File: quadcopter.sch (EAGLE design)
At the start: 66 parts, among them J1 ISP, J4 SIP-10_TH-254X10, M1 MOTOR_PADS, M2 MOTOR_PADS, M3 MOTOR_PADS, M4 MOTOR_PADS, U1 ATMEGA128RFA1, Y1 16MHz

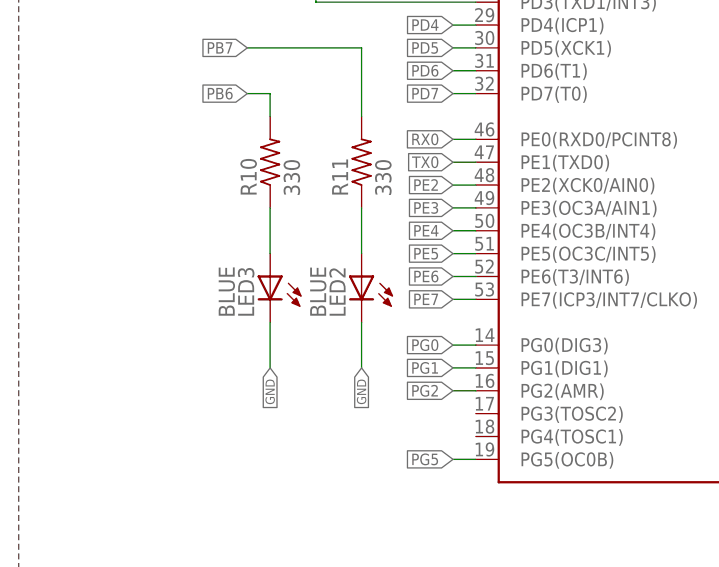
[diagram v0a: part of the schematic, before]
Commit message: Version before generating cam
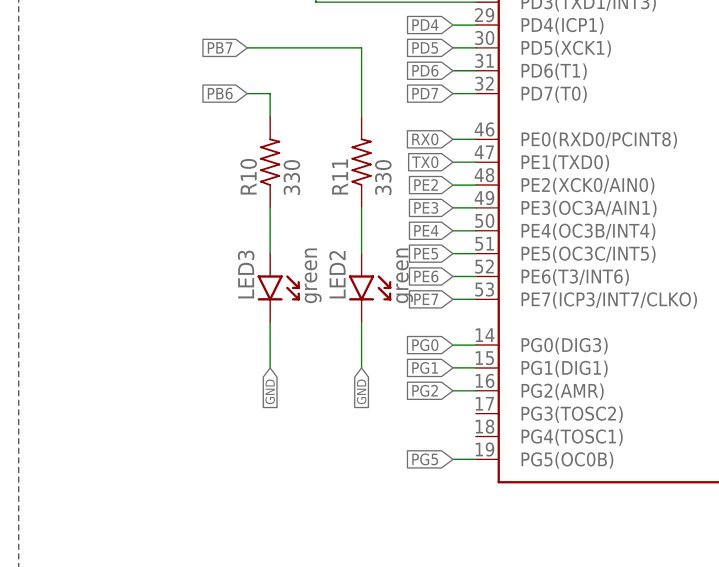
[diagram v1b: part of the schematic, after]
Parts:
- LED2, LED3: value BLUE -> green; device Yueqi Wang-Lab2:LED5MM -> quadparts_prebuilt:DIODE-LED_SMD-2012-0805-GREEN
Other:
- moved on the sheet: LED2, LED3
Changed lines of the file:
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@@
 <part name="JP9" library="quadparts_prebuilt" deviceset="FTDI_BASIC" device="PTH" value="FTDI"/>
 <part name="C16" library="quadparts_prebuilt" deviceset="CAPACITOR-NP_" device="SMD-2012-0805_CERAMIC-0.1UF" value="0.1uF"/>
-<part name="LED2" library="Yueqi Wang-Lab2" deviceset="LED" device="5MM" value="BLUE"/>
+<part name="LED2" library="quadparts_prebuilt" deviceset="DIODE-LED_" device="SMD-2012-0805-GREEN" value="green"/>
 <part name="C17" library="quadparts_prebuilt" deviceset="CAPACITOR-NP_" device="SMD-2012-0805_CERAMIC-0.75PF" value="0.75pF"/>
-<part name="LED3" library="Yueqi Wang-Lab2" deviceset="LED" device="5MM" value="BLUE"/>
+<part name="LED3" library="quadparts_prebuilt" deviceset="DIODE-LED_" device="SMD-2012-0805-GREEN" value="green"/>
 <part name="R10" library="quadparts_prebuilt" deviceset="RESISTOR_" device="SMD-2012-0805-330" value="330"/>
 <part name="R11" library="quadparts_prebuilt" deviceset="RESISTOR_" device="SMD-2012-0805-330" value="330"/>
@@
 <instance part="JP9" gate="G$1" x="38.1" y="45.72" rot="MR180"/>
 <instance part="C16" gate="G$1" x="58.42" y="50.8" rot="R90"/>
-<instance part="LED2" gate="G$1" x="-83.82" y="-129.54" rot="MR0"/>
+<instance part="LED2" gate="G$1" x="-83.82" y="-129.54" rot="MR270"/>
 <instance part="C17" gate="G$1" x="53.34" y="-81.28" rot="MR180"/>
-<instance part="LED3" gate="G$1" x="-93.98" y="-129.54" rot="MR0"/>
+<instance part="LED3" gate="G$1" x="-93.98" y="-129.54" rot="MR270"/>
 <instance part="R10" gate="G$1" x="-93.98" y="-116.84" rot="R90"/>
 <instance part="R11" gate="G$1" x="-83.82" y="-116.84" rot="R90"/>
